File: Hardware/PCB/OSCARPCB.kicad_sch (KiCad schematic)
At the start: 1 part

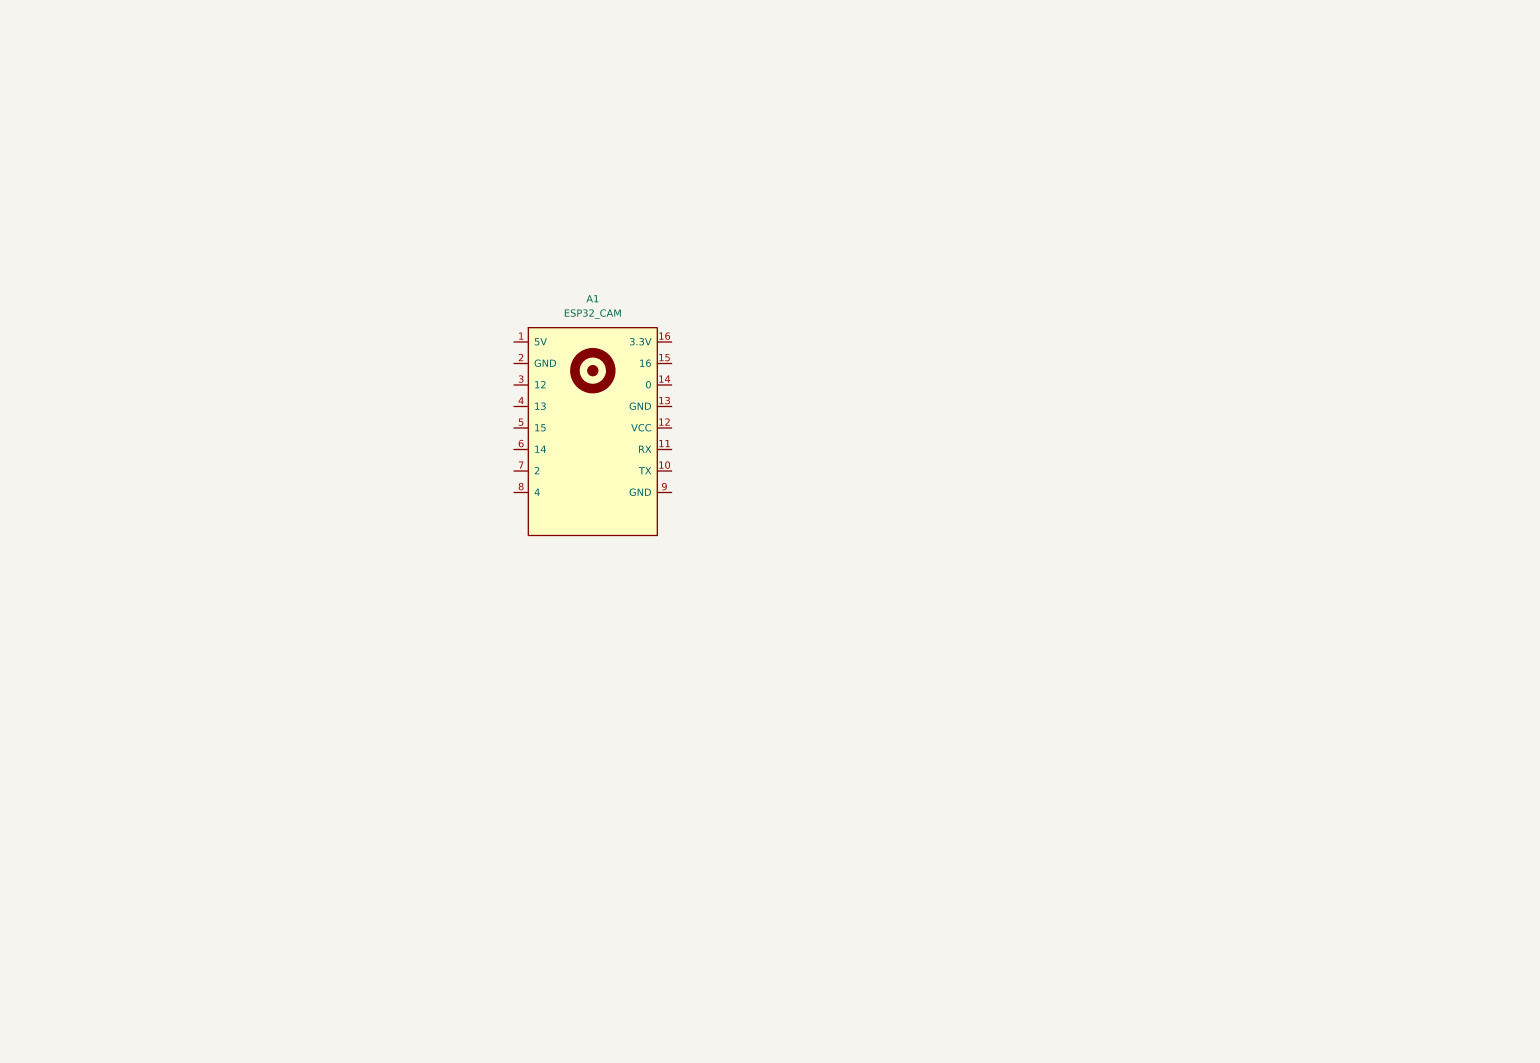
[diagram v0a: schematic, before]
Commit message: Started PCB schematic
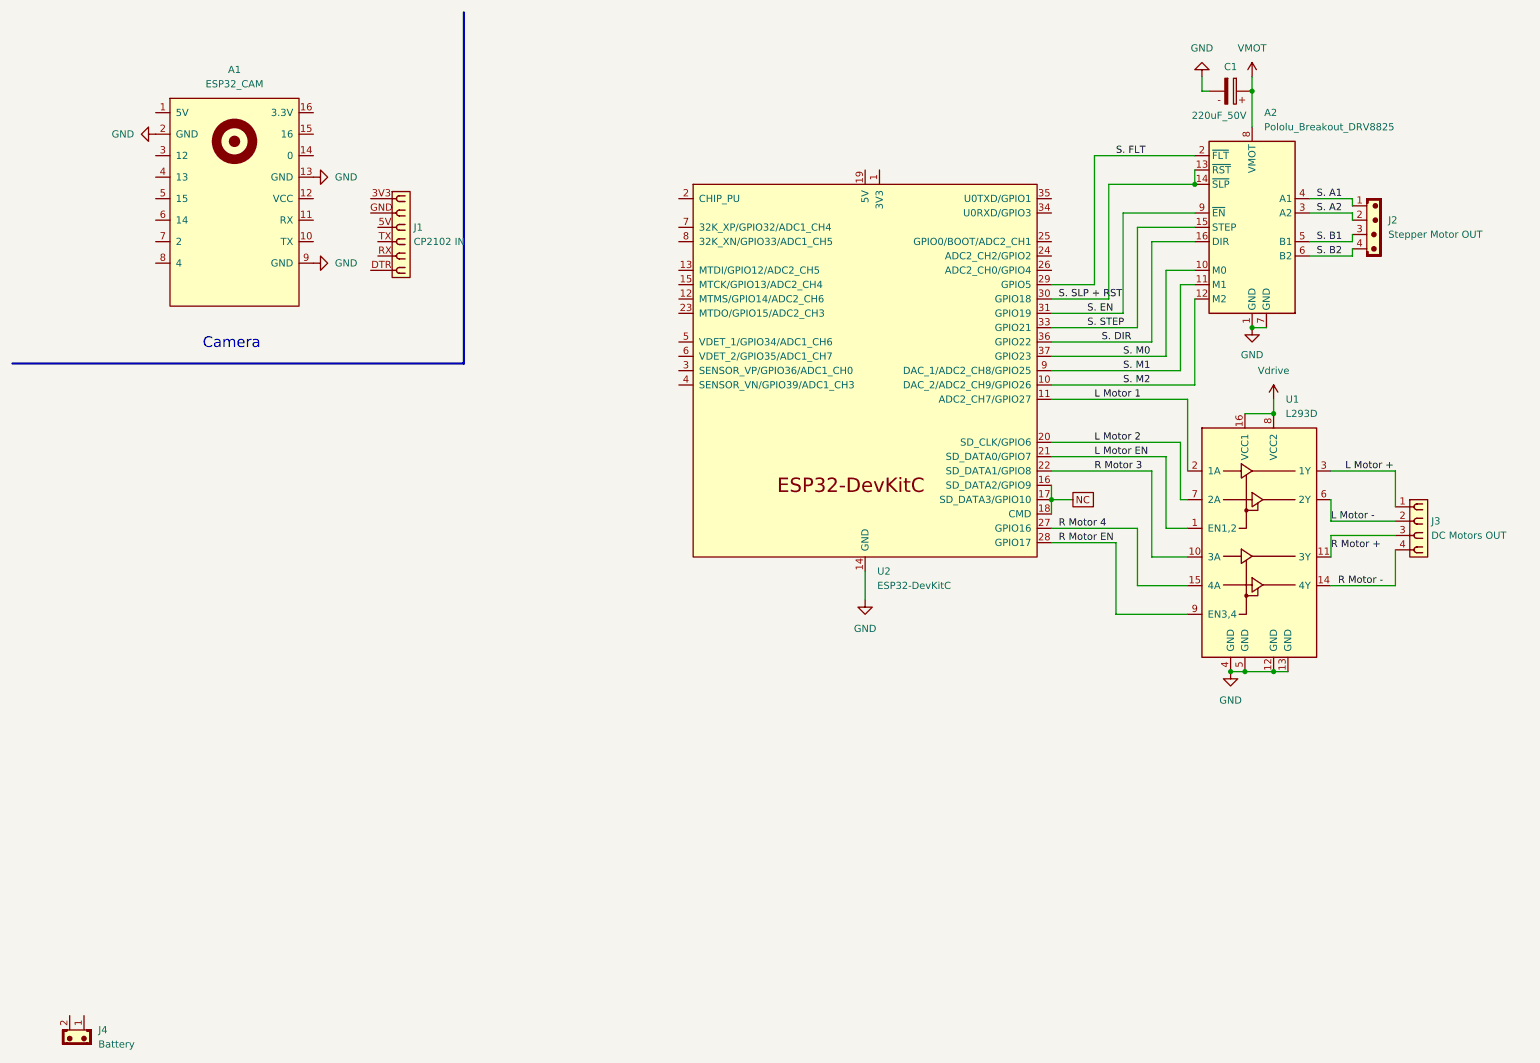
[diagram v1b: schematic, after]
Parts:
- added A2: Pololu_Breakout_DRV8825, Module:Pololu_Breakout-16_15.2x20.3mm, symbol Driver_Motor:Pololu_Breakout_DRV8825
- added C1: 220uF_50V, Capacitor_THT:CP_Radial_D10.0mm_P5.00mm, symbol PCM_SL_Capacitors:220uF_50V
- added J1: CP2102 IN, Connector_PinSocket_2.54mm:PinSocket_1x06_P2.54mm_Vertical, symbol PCM_SL_Pin_Headers:PINHD_1x6_Female
- added J2: Stepper Motor OUT, Connector_JST:JST_EH_B4B-EH-A_1x04_P2.50mm_Vertical, symbol PCM_SL_Connectors:JST_04
- added J3: DC Motors OUT, Connector_PinSocket_2.54mm:PinSocket_1x04_P2.54mm_Vertical, symbol PCM_SL_Pin_Headers:PINHD_1x4_Female
- added J4: Battery, Connector_JST:JST_EH_B2B-EH-A_1x02_P2.50mm_Vertical, symbol PCM_SL_Connectors:JST_02
- added U1: L293D, Package_DIP:DIP-16_W7.62mm, symbol Driver_Motor:L293D
- added U2: ESP32-DevKitC, PCM_Espressif:ESP32-DevKitC, symbol PCM_Espressif:ESP32-DevKitC
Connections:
- net GND: now reaches A1.13 (GND)
- net GND: now also A1.2 (GND), A1.9 (GND), A2.1 (GND), A2.7 (GND), C1.2, U1.12 (GND), U1.13 (GND), U1.4 (GND), U1.5 (GND), U2.14 (GND), U2.32 (GND), U2.38 (GND)
- new net L Motor +: J3.1, U1.3 (1Y)
- new net L Motor -: J3.2, U1.6 (2Y)
- new net L Motor 1: U1.2 (1A), U2.11 (ADC2_CH7/GPIO27)
- new net L Motor 2: U1.7 (2A), U2.20 (SD_CLK/GPIO6)
- new net L Motor EN: U1.1 (EN1,2), U2.21 (SD_DATA0/GPIO7)
- new net NC: U2.16 (SD_DATA2/GPIO9), U2.17 (SD_DATA3/GPIO10), U2.18 (CMD)
- new net R Motor +: J3.3, U1.11 (3Y)
- new net R Motor -: J3.4, U1.14 (4Y)
- new net R Motor 3: U1.10 (3A), U2.22 (SD_DATA1/GPIO8)
- new net R Motor 4: U1.15 (4A), U2.27 (GPIO16)
- new net R Motor EN: U1.9 (EN3,4), U2.28 (GPIO17)
- new net S. A1: A2.4 (A1), J2.1
- new net S. A2: A2.3 (A2), J2.2
- new net S. B1: A2.5 (B1), J2.3
- new net S. B2: A2.6 (B2), J2.4
- new net S. DIR: A2.16 (DIR), U2.36 (GPIO22)
- new net S. EN: A2.9 (~{EN}), U2.31 (GPIO19)
- new net S. FLT: A2.2 (~{FLT}), U2.29 (GPIO5)
- new net S. M0: A2.10 (M0), U2.37 (GPIO23)
- new net S. M1: A2.11 (M1), U2.9 (DAC_1/ADC2_CH8/GPIO25)
- new net S. M2: A2.12 (M2), U2.10 (DAC_2/ADC2_CH9/GPIO26)
- new net S. SLP + RST: A2.13 (~{RST}), A2.14 (~{SLP}), U2.30 (GPIO18)
- new net S. STEP: A2.15 (STEP), U2.33 (GPIO21)
- new net VMOT: A2.8 (VMOT), C1.1
- new net Vdrive: U1.16 (VCC1), U1.8 (VCC2)
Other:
- note added: "Camera"
- moved on the sheet: A1
